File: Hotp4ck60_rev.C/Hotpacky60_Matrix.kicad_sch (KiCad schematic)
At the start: 127 parts

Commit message: README 수정
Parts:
- D1, D10, D11, D12, D13, D14, D15, D16, D17, D18, D19, D2, D20, D21, D22, D23, D24, D25, D26, D27, D28, D29, D3, D30, D31, D32, D33, D34, D35, D36, D37, D38, D39, D4, D40, D41, D42, D43, D44, D45, D46, D47, D48, D49, D5, D50, D51, D52, D53, D54, D55, D56, D57, D58, D59, D6, D60, D61, D62, D63, D7, D8, D9: LCSC (none) -> C2128

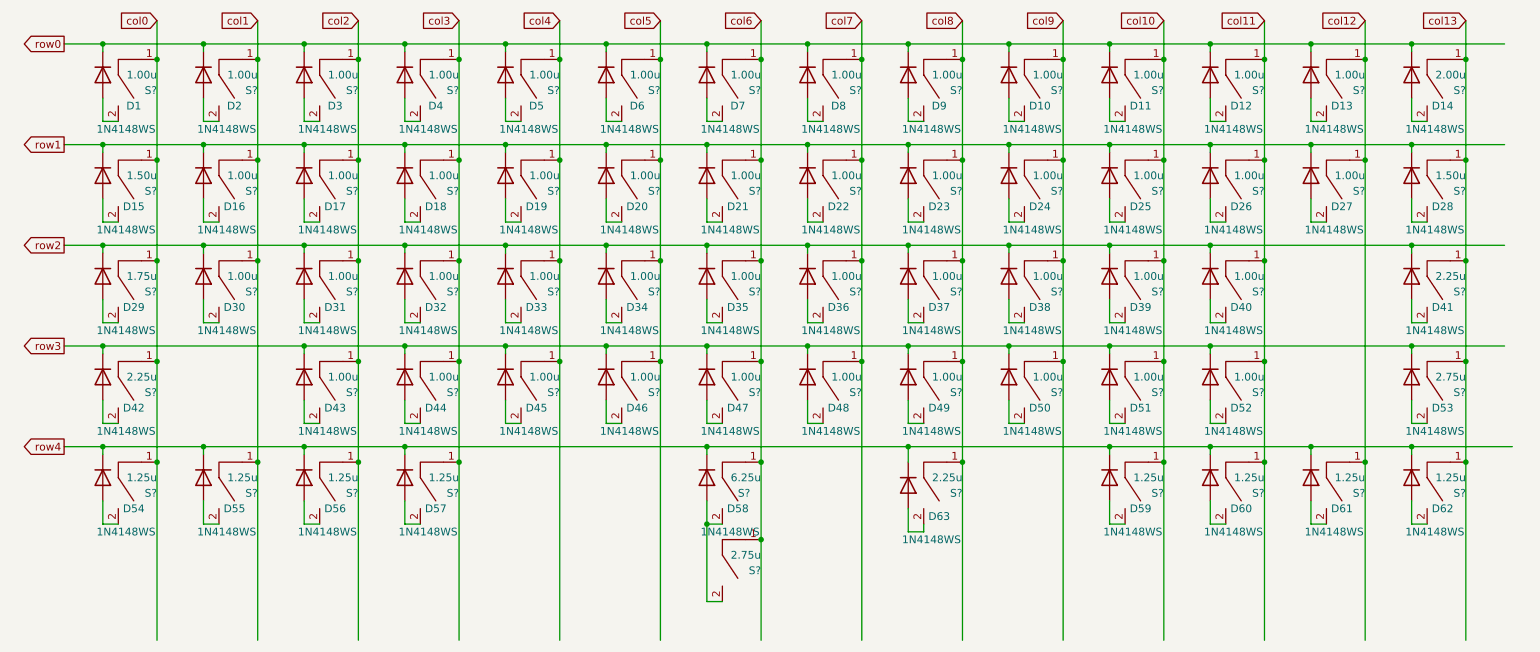
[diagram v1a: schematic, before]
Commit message: rev.C neocore
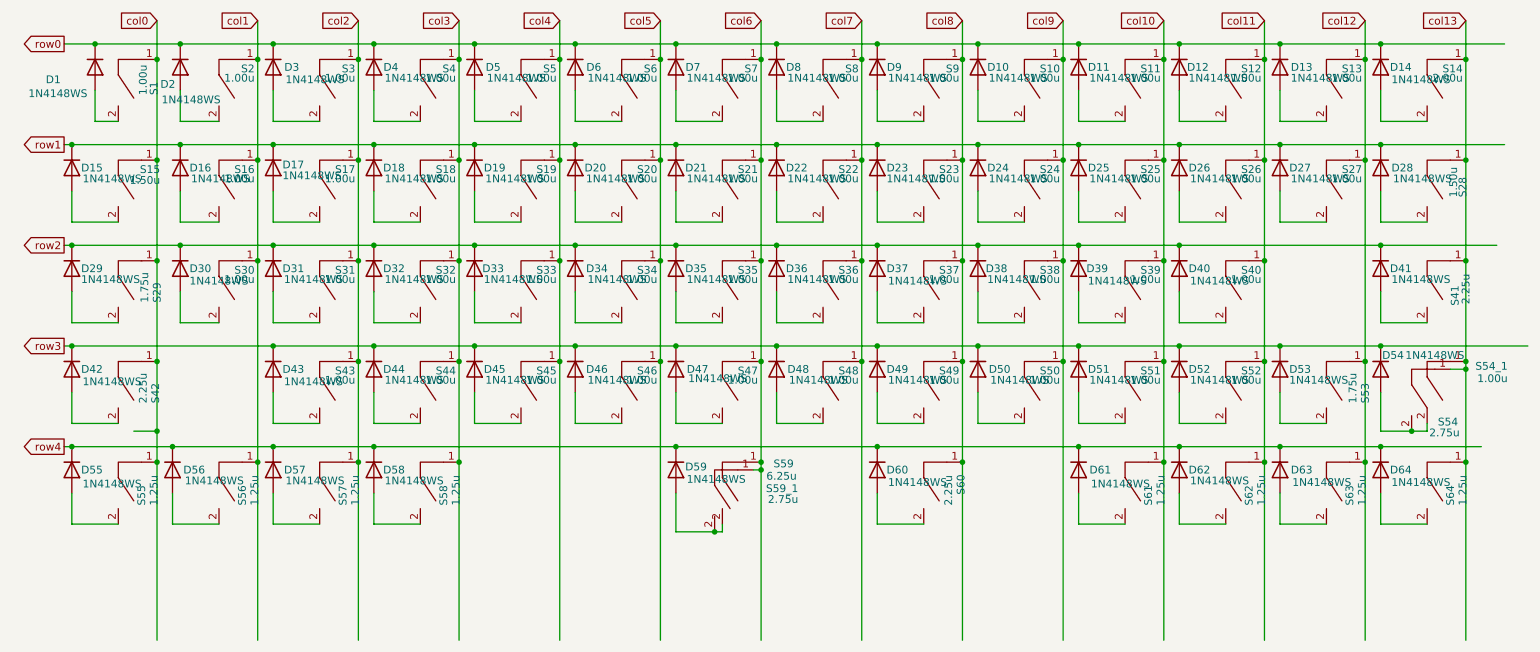
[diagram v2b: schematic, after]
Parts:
- removed S? (x45): 1.00u, Switch_Keyboard_Cherry_MX:SW_Cherry_MX_PCB_1.00u, symbol mx1a-simple:MX1A
- removed S? (x7): 1.25u, Switch_Keyboard_Cherry_MX:SW_Cherry_MX_PCB_1.25u, symbol mx1a-simple:MX1A
- removed S?: 2.00u, Switch_Keyboard_Cherry_MX:SW_Cherry_MX_PCB_2.00u, symbol mx1a-simple:MX1A
- removed S?: 1.50u, Switch_Keyboard_Cherry_MX:SW_Cherry_MX_PCB_1.50u, symbol mx1a-simple:MX1A
- added D53: 1N4148WS, Diode_SMD:D_SOD-323, symbol Diode:1N4148WS
- added S10, S11, S12, S13, S16, S17, S18, S19, S2, S20, S21, S22, S23, S24, S25, S26, S27, S3, S30, S31, S32, S33, S34, S35, S36, S37, S38, S39, S4, S40, S43, S44, S45, S46, S47, S48, S49, S5, S50, S51, S52, S54_1, S6, S7, S8, S9: 1.00u, Switch_Keyboard_Cherry_MX:SW_Cherry_MX_PCB_1.00u, symbol mx1a-simple:MX1A
- added S14: 2.00u, Switch_Keyboard_Cherry_MX:SW_Cherry_MX_PCB_2.00u, symbol mx1a-simple:MX1A
- added S28: 1.50u, Switch_Keyboard_Cherry_MX:SW_Cherry_MX_PCB_1.50u, symbol mx1a-simple:MX1A
- added S53: 1.75u, Switch_Keyboard_Cherry_MX:SW_Cherry_MX_PCB_1.75u, symbol mx1a-simple:MX1A
- added S56, S57, S58, S61, S62, S63, S64: 1.25u, Switch_Keyboard_Cherry_MX:SW_Cherry_MX_PCB_1.25u, symbol mx1a-simple:MX1A
- gave numbers to parts that had none: 10
- renumbered D53 to D54, D54 to D55, D55 to D56, D56 to D57, D57 to D58, D58 to D59, D63 to D60, D59 to D61, D60 to D62, D61 to D63, D62 to D64
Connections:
- net col0: now also S1.1
- net col1: now also S16.1, S2.1, S30.1, S56.1
- net col10: now also S11.1, S25.1, S39.1, S51.1, S61.1
- net col11: now also S12.1, S26.1, S40.1, S52.1, S62.1
- net col12: now also S13.1, S27.1, S53.1, S63.1
- net col13: now also S14.1, S28.1, S54_1.1, S64.1
- net col2: now also S17.1, S3.1, S31.1, S43.1, S57.1; no longer S1.1
- net col3: now also S18.1, S32.1, S4.1, S44.1, S58.1
- net col4: now also S19.1, S33.1, S45.1, S5.1
- net col5: now also S20.1, S34.1, S46.1, S6.1
- net col6: now also S21.1, S35.1, S47.1, S7.1
- net col7: now also S22.1, S36.1, S48.1, S8.1
- net col8: now also S23.1, S37.1, S49.1, S9.1
- net col9: now also S10.1, S24.1, S38.1, S50.1
- net row3: now also D53.1 (K)
- net at D56.2 (A): now also S56.2
- net at D64.2 (A): now also S64.2
- net at D57.2 (A): now also S57.2
- net at D25.2 (A): now also S25.2
- net at D2.2 (A): now also S2.2
- net at D27.2 (A): now also S27.2
- net at D45.2 (A): now also S45.2
- net at D36.2 (A): now also S36.2
- net at D63.2 (A): now also S63.2
- net at D23.2 (A): now also S23.2
- net at D14.2 (A): now also S14.2
- net at D8.2 (A): now also S8.2
- net at D35.2 (A): now also S35.2
- net at D26.2 (A): now also S26.2
- net at D52.2 (A): now also S52.2
- net at D5.2 (A): now also S5.2
- net at D46.2 (A): now also S46.2
- net at D50.2 (A): now also S50.2
- net at D43.2 (A): now also S43.2; no longer S1.2
- net at D34.2 (A): now also S34.2
- net at D6.2 (A): now also S6.2
- net at D38.2 (A): now also S38.2
- net at D32.2 (A): now also S32.2
- net at D4.2 (A): now also S4.2
- net at D11.2 (A): now also S11.2
- net at D62.2 (A): now also S62.2
- net at D51.2 (A): now also S51.2
- net at D3.2 (A): now also S3.2
- net at D21.2 (A): now also S21.2
- net at D30.2 (A): now also S30.2
- net at D49.2 (A): now also S49.2
- net at D39.2 (A): now also S39.2
- net at D33.2 (A): now also S33.2
- net at D13.2 (A): now also S13.2
- net at D48.2 (A): now also S48.2
- net at D54.2 (A), S54.2: now also S54_1.2
- net at D28.2 (A): now also S28.2
- net at D7.2 (A): now also S7.2
- net at D22.2 (A): now also S22.2
- net at D1.2 (A): now also S1.2
- net at D19.2 (A): now also S19.2
- net at D40.2 (A): now also S40.2
- net at D47.2 (A): now also S47.2
- net at D9.2 (A): now also S9.2
- net at D44.2 (A): now also S44.2
- net at D58.2 (A): now also S58.2
- net at D20.2 (A): now also S20.2
- net at D24.2 (A): now also S24.2
- net at D16.2 (A): now also S16.2
- net at D18.2 (A): now also S18.2
- net at D12.2 (A): now also S12.2
- net at D61.2 (A): now also S61.2
- net at D37.2 (A): now also S37.2
- net at D31.2 (A): now also S31.2
- net at D17.2 (A): now also S17.2
- net at D10.2 (A): now also S10.2
- new net: D53.2 (A), S53.2
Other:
- moved on the sheet: D1, D10, D11, D12, D13, D14, D15, D16, D17, D18, D19, D2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
